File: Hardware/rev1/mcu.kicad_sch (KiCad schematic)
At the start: 18 parts, among them J1 Conn_ARM_JTAG_SWD_10, SW1 SW_Push, U1 STM32F103C8Tx, U3 MS5607-02BA, U4 W25Q128JVS, Y1 16MHz

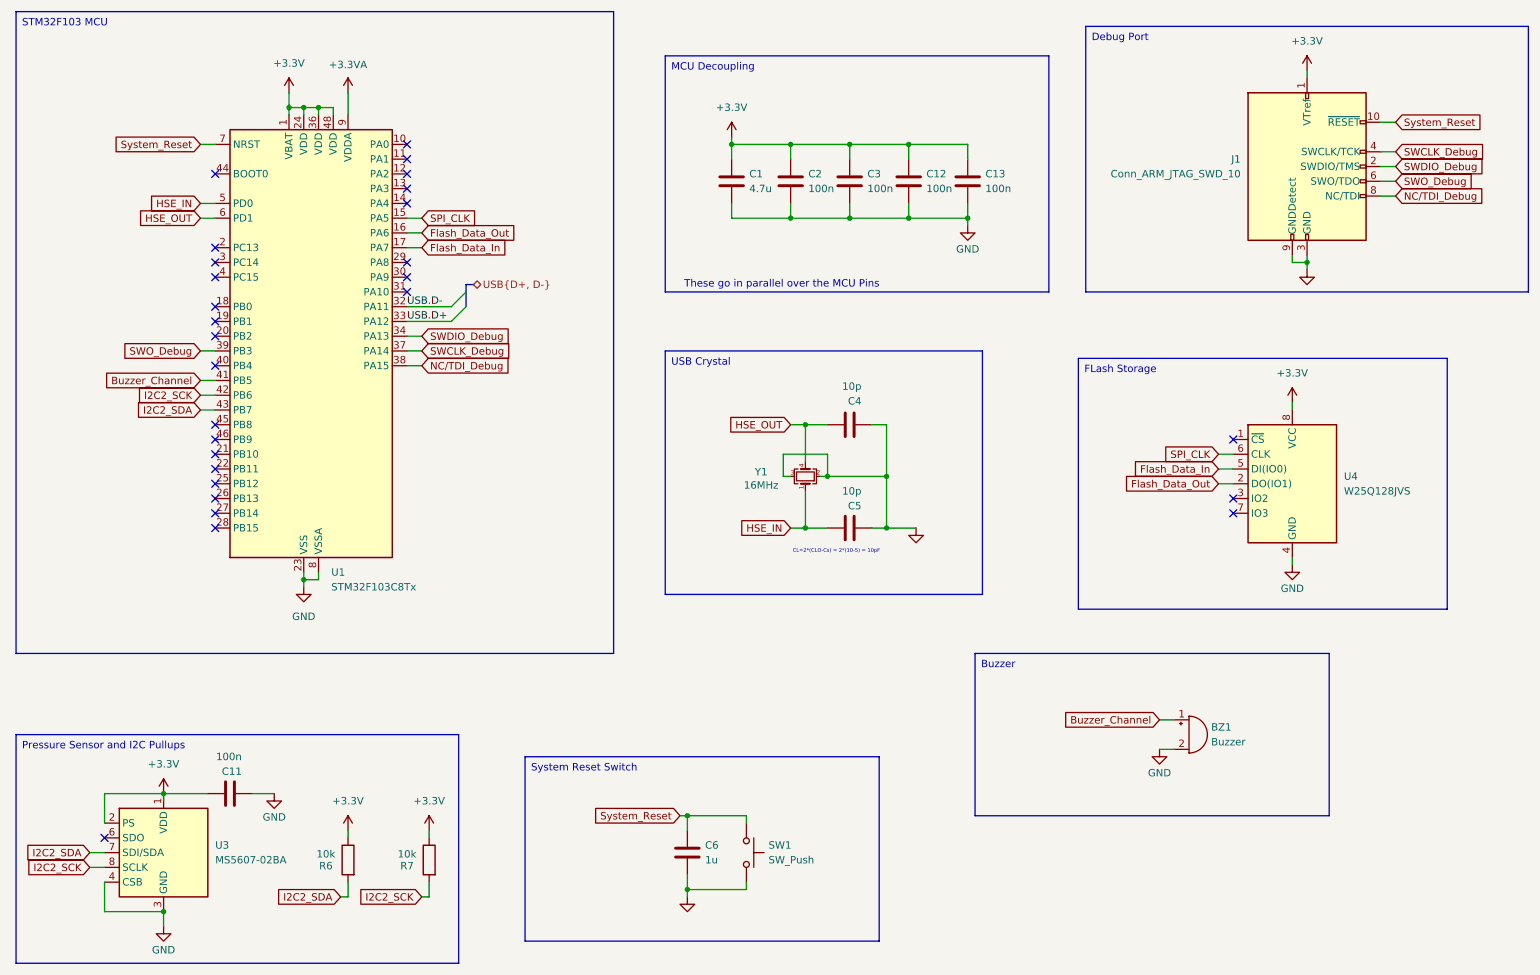
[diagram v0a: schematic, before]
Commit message: i dont know what the local change is
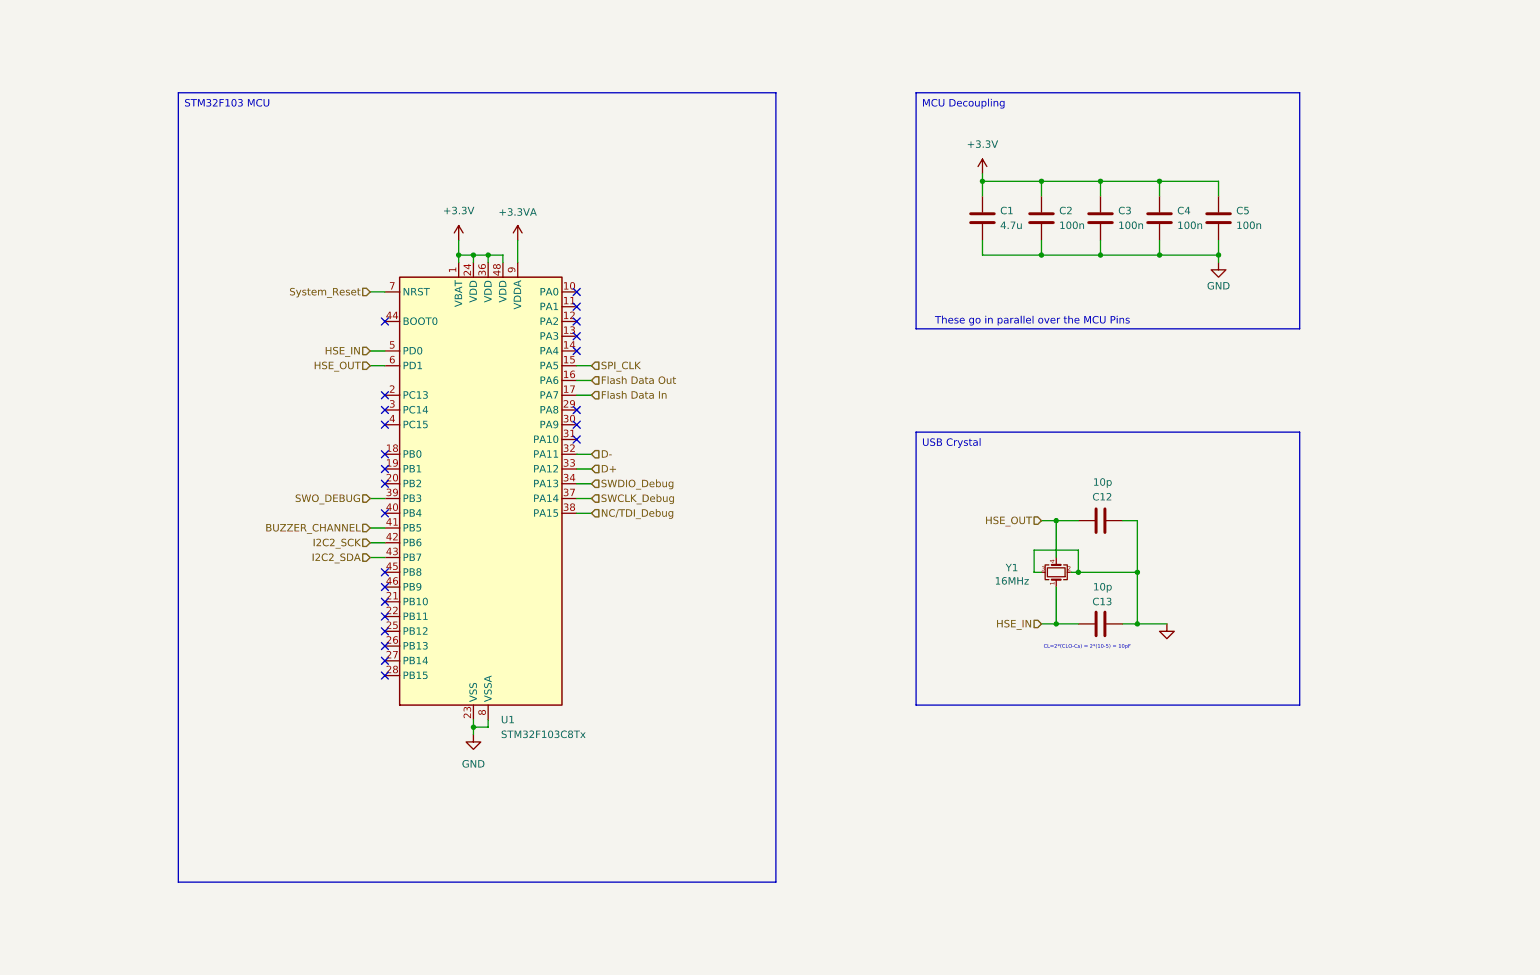
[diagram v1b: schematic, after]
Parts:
- removed BZ1: Buzzer, symbol Device:Buzzer
- removed C11: 100n, symbol Device:C
- removed C6: 1u, symbol Device:C
- removed J1: Conn_ARM_JTAG_SWD_10, symbol Connector:Conn_ARM_JTAG_SWD_10
- removed R6, R7: 10k, Resistor_SMD:R_0402_1005Metric, symbol Device:R
- removed SW1: SW_Push, symbol Switch:SW_Push
- removed U3: MS5607-02BA, Package_LGA:LGA-8_3x5mm_P1.25mm, symbol Sensor_Pressure:MS5607-02BA
- removed U4: W25Q128JVS, Package_SO:SOIC-8_5.23x5.23mm_P1.27mm, symbol Memory_Flash:W25Q128JVS
- C12, C13: value 100n -> 10p; footprint (none) -> Capacitor_SMD:C_0402_1005Metric
- C4, C5: value 10p -> 100n; footprint Capacitor_SMD:C_0402_1005Metric -> (none)
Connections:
- net +3.3V: now also C4.1, C5.1; no longer C12.1, C13.1
- net HSE_IN: now also C13.1; no longer C5.1
- net HSE_OUT: now also C12.1; no longer C4.1
- net Buzzer_Channel renamed BUZZER_CHANNEL
- net Flash_Data_In renamed Flash Data In
- net Flash_Data_Out renamed Flash Data Out
- net SWO_Debug renamed SWO_DEBUG
- net USB.D+ renamed D+
- net USB.D- renamed D-
- no-connect marks 28 -> 24
